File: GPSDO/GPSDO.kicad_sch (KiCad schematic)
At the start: 37 parts, among them J1 analog, J2 Conn_01x03_Pin, J3 USB_B_Mini, J4 1PPSin, SW1 RST#, U1 FT230XS, U2 CH32V003FxPx, U3 TLV9061xDBV, Y2 24 MHz Farnell 4165823

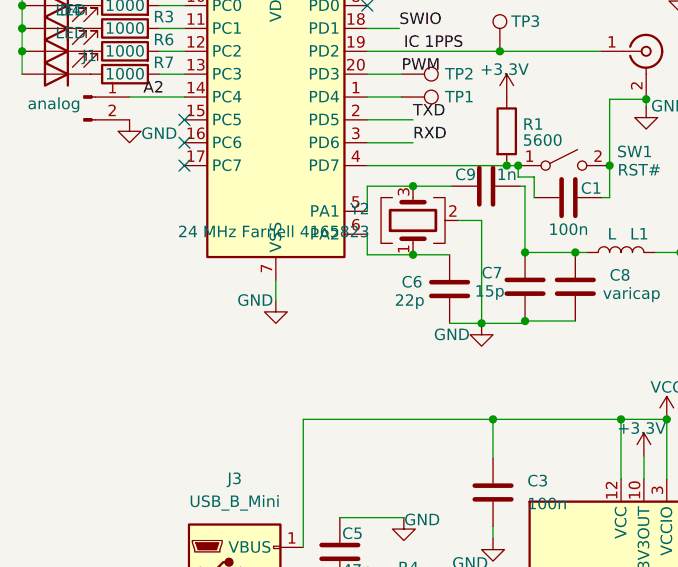
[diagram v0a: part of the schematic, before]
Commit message: 3D model
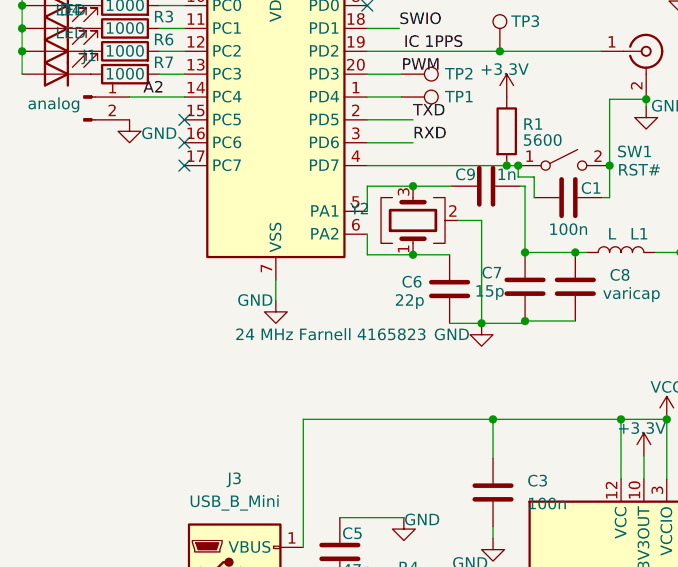
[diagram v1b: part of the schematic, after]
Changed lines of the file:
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@@
 		(in_pos_files yes)
 		(dnp no)
-		(fields_autoplaced yes)
 		(property "Reference" "Y2"
 			(at 88.9 60.1979 90)
@@
 		)
 		(property "Value" "24 MHz Farnell 4165823"
-			(at 88.9 62.7379 90)
+			(at 95.25 74.168 90)
 			(show_name no)
 			(do_not_autoplace no)
